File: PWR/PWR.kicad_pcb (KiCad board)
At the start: 2 copper layers, 71.6 x 70.1 mm, 21 parts, among them J1 +12v, P1 +5v, P2 GND, SW1 SPDT

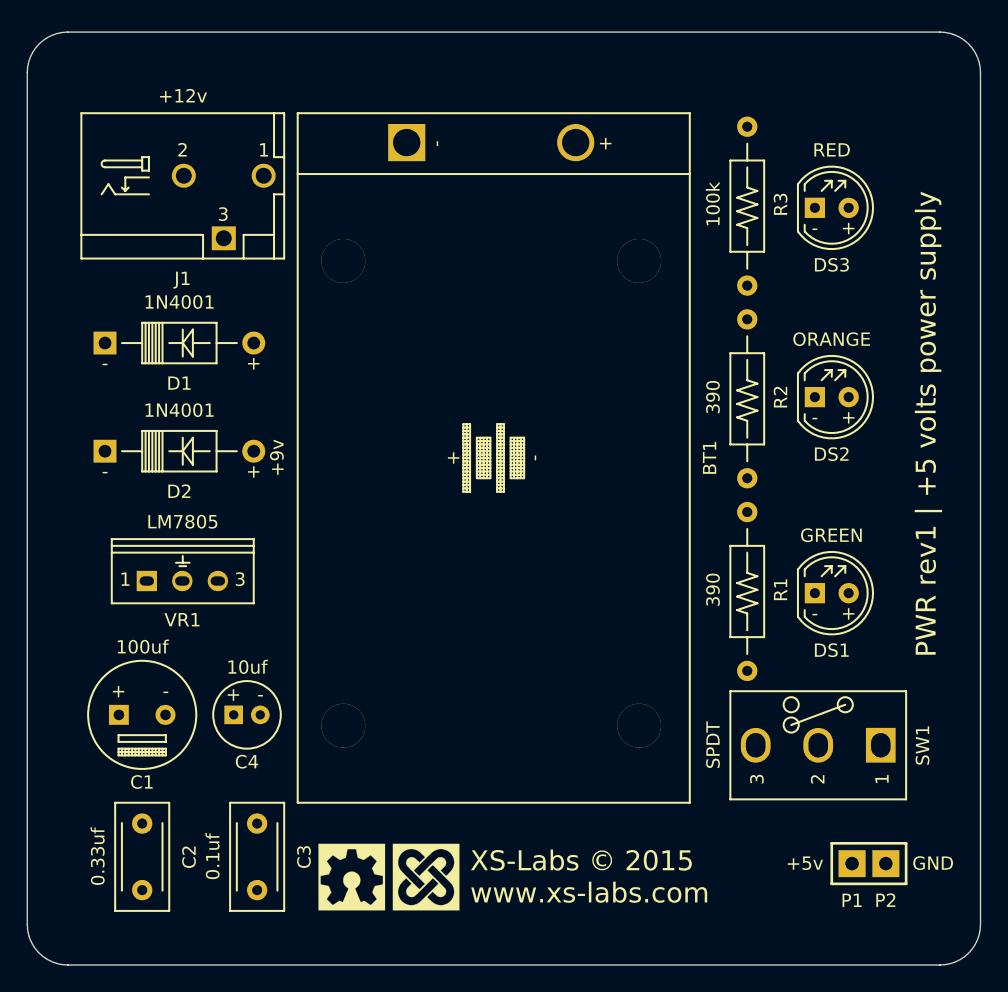
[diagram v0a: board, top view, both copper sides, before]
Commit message: PCB edges.
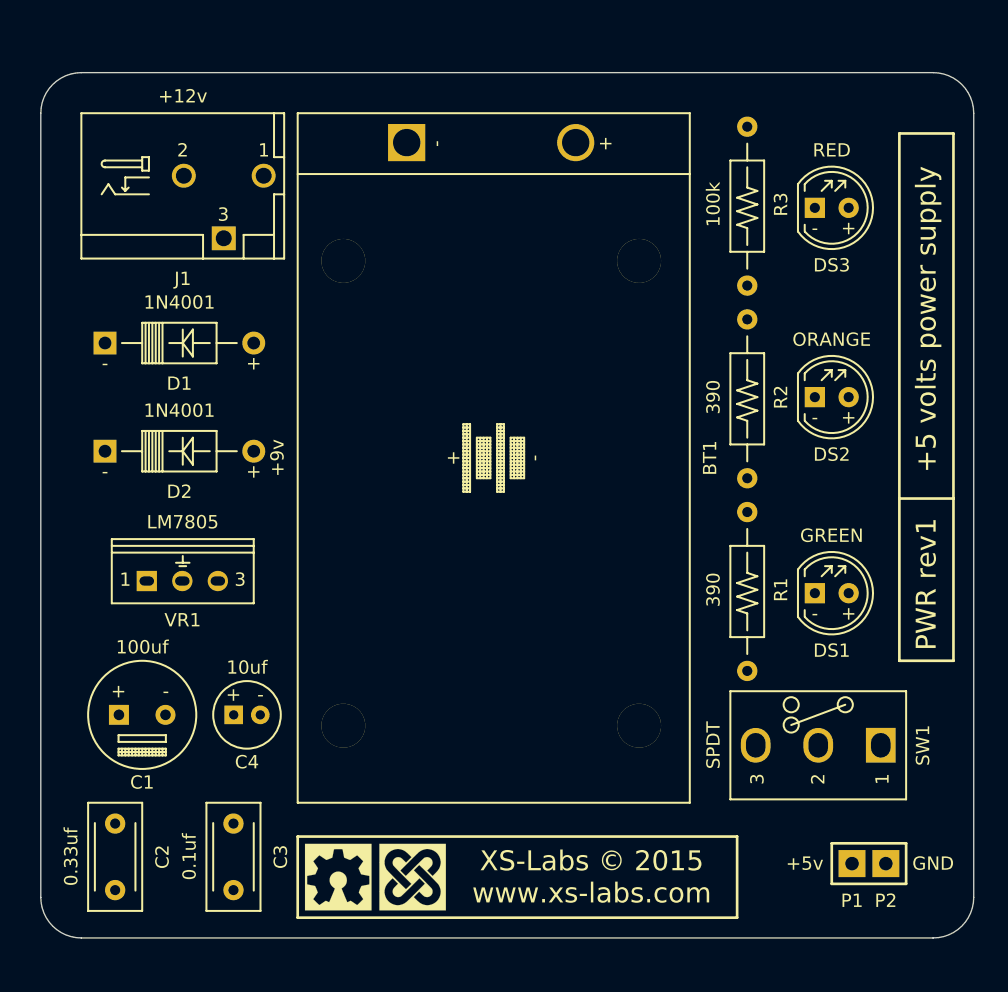
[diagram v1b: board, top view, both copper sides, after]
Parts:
- moved C2 2.03 mm to (105.7, 124.5)
- moved C3 1.78 mm to (114.6, 124.5)
- moved G*** 1.02 mm to (128.0, 126.0)
- moved G*** 1.02 mm to (122.4, 126.0)
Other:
- board size 71.6 x 70.1 mm -> 70.1 x 65 mm
- board text added: "+5 volts power supply"
- board text added: "PWR rev1"
- board text removed: "PWR rev1 | +5 volts power supply"
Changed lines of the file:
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@@
     (links 26)
     (no_connects 26)
-    (area 99.009999 62.433999 170.738001 132.638001)
+    (area 100.025999 65.481999 170.230001 130.606001)
     (thickness 1.6)
-    (drawings 14)
+    (drawings 26)
     (tracks 0)
     (zones 0)
@@
   )
   (module XS:Logo-OWH (layer F.Cu)
-    (at 123.444 125.984)
+    (at 122.428 125.984)
     (fp_text reference G*** (at 0 0) (layer F.SilkS) hide
       (effects (font (thickness 0.3)))
@@
   )
   (module XS:Logo-XS (layer F.Cu)
-    (at 129.032 125.984)
+    (at 128.016 125.984)
     (fp_text reference G*** (at 0 0) (layer F.SilkS) hide
       (effects (font (thickness 0.3)))
@@
   )
   (module XS:Capacitor-Murata-RCE-Series-5mm (layer F.Cu)
-    (at 107.696 124.46 90)
+    (at 105.664 124.46 90)
     (fp_text reference C2 (at 0 3.556 90) (layer F.SilkS)
       (effects (font (size 1 1) (thickness 0.15)))
@@
   )
   (module XS:Capacitor-Murata-RCE-Series-5mm (layer F.Cu)
-    (at 116.332 124.46 90)
+    (at 114.554 124.46 90)
     (fp_text reference C3 (at 0 3.556 90) (layer F.SilkS)
       (effects (font (size 1 1) (thickness 0.15)))
@@
       (xy 14.986 -14.986)) (layer B.SilkS) (width 0.01))
   )
+  (gr_line (start 167.132 130.556) (end 103.124 130.556) (angle 90) (layer Edge.Cuts) (width 0.1))
+  (gr_line (start 170.18 127.508) (end 170.18 68.58) (angle 90) (layer Edge.Cuts) (width 0.1))
+  (gr_line (start 103.124 65.532) (end 167.132 65.532) (angle 90) (layer Edge.Cuts) (width 0.1))
+  (gr_line (start 100.076 127.508) (end 100.076 68.58) (angle 90) (layer Edge.Cuts) (width 0.1))
+  (gr_line (start 168.656 70.104) (end 168.656 97.536) (angle 90) (layer F.SilkS) (width 0.2))
+  (gr_line (start 164.592 70.104) (end 164.592 97.536) (angle 90) (layer F.SilkS) (width 0.2))
+  (gr_line (start 168.656 70.104) (end 164.592 70.104) (angle 90) (layer F.SilkS) (width 0.2))
+  (gr_text "+5 volts power supply" (at 166.624 84.074 90) (layer F.SilkS)
+    (effects (font (size 1.5 1.5) (thickness 0.3)))
+  )
+  (gr_line (start 164.592 109.728) (end 164.592 97.536) (angle 90) (layer F.SilkS) (width 0.2))
+  (gr_line (start 168.656 97.536) (end 168.656 109.728) (angle 90) (layer F.SilkS) (width 0.2))
+  (gr_line (start 164.592 97.536) (end 168.656 97.536) (angle 90) (layer F.SilkS) (width 0.2))
+  (gr_line (start 164.592 109.728) (end 168.656 109.728) (angle 90) (layer F.SilkS) (width 0.2))
+  (gr_line (start 152.4 122.936) (end 119.38 122.936) (angle 90) (layer F.SilkS) (width 0.2))
+  (gr_line (start 152.4 129.032) (end 152.4 122.936) (angle 90) (layer F.SilkS) (width 0.2))
+  (gr_line (start 119.38 129.032) (end 152.4 129.032) (angle 90) (layer F.SilkS) (width 0.2))
+  (gr_line (start 119.38 122.936) (end 119.38 129.032) (angle 90) (layer F.SilkS) (width 0.2))
   (gr_line (start 159.512 126.492) (end 159.512 123.444) (angle 90) (layer F.SilkS) (width 0.2))
   (gr_line (start 165.1 126.492) (end 159.512 126.492) (angle 90) (layer F.SilkS) (width 0.2))
   (gr_line (start 165.1 123.444) (end 165.1 126.492) (angle 90) (layer F.SilkS) (width 0.2))
   (gr_line (start 159.512 123.444) (end 165.1 123.444) (angle 90) (layer F.SilkS) (width 0.2))
-  (gr_text "PWR rev1 | +5 volts power supply" (at 166.624 109.474 90) (layer F.SilkS)
+  (gr_text "PWR rev1" (at 166.624 108.966 90) (layer F.SilkS)
     (effects (font (size 1.5 1.5) (thickness 0.3)) (justify left))
   )
-  (gr_line (start 99.06 65.532) (end 99.06 129.54) (angle 90) (layer Edge.Cuts) (width 0.1))
-  (gr_line (start 167.64 132.588) (end 102.108 132.588) (angle 90) (layer Edge.Cuts) (width 0.1))
-  (gr_line (start 170.688 65.532) (end 170.688 129.54) (angle 90) (layer Edge.Cuts) (width 0.1))
-  (gr_line (start 102.108 62.484) (end 167.64 62.484) (angle 90) (layer Edge.Cuts) (width 0.1))
-  (gr_arc (start 102.108 129.54) (end 102.108 132.588) (angle 90) (layer Edge.Cuts) (width 0.1))
-  (gr_arc (start 167.64 129.54) (end 170.688 129.54) (angle 90) (layer Edge.Cuts) (width 0.1))
-  (gr_arc (start 167.64 65.532) (end 167.64 62.484) (angle 90) (layer Edge.Cuts) (width 0.1))
-  (gr_arc (start 102.108 65.532) (end 99.06 65.532) (angle 90) (layer Edge.Cuts) (width 0.1))
-  (gr_text "XS-Labs © 2015\nwww.xs-labs.com" (at 132.334 125.984) (layer F.SilkS)
-    (effects (font (size 1.5 1.5) (thickness 0.3)) (justify left))
+  (gr_arc (start 103.124 127.508) (end 103.124 130.556) (angle 90) (layer Edge.Cuts) (width 0.1))
+  (gr_arc (start 167.132 127.508) (end 170.18 127.508) (angle 90) (layer Edge.Cuts) (width 0.1))
+  (gr_arc (start 167.132 68.58) (end 167.132 65.532) (angle 90) (layer Edge.Cuts) (width 0.1))
+  (gr_arc (start 103.124 68.58) (end 100.076 68.58) (angle 90) (layer Edge.Cuts) (width 0.1))
+  (gr_text "XS-Labs © 2015\nwww.xs-labs.com" (at 141.478 125.984) (layer F.SilkS)
+    (effects (font (size 1.5 1.5) (thickness 0.3)))
   )
 )
